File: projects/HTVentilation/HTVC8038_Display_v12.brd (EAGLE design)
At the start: 80.6 x 58.7 mm, 34 parts, among them IC1 7805T

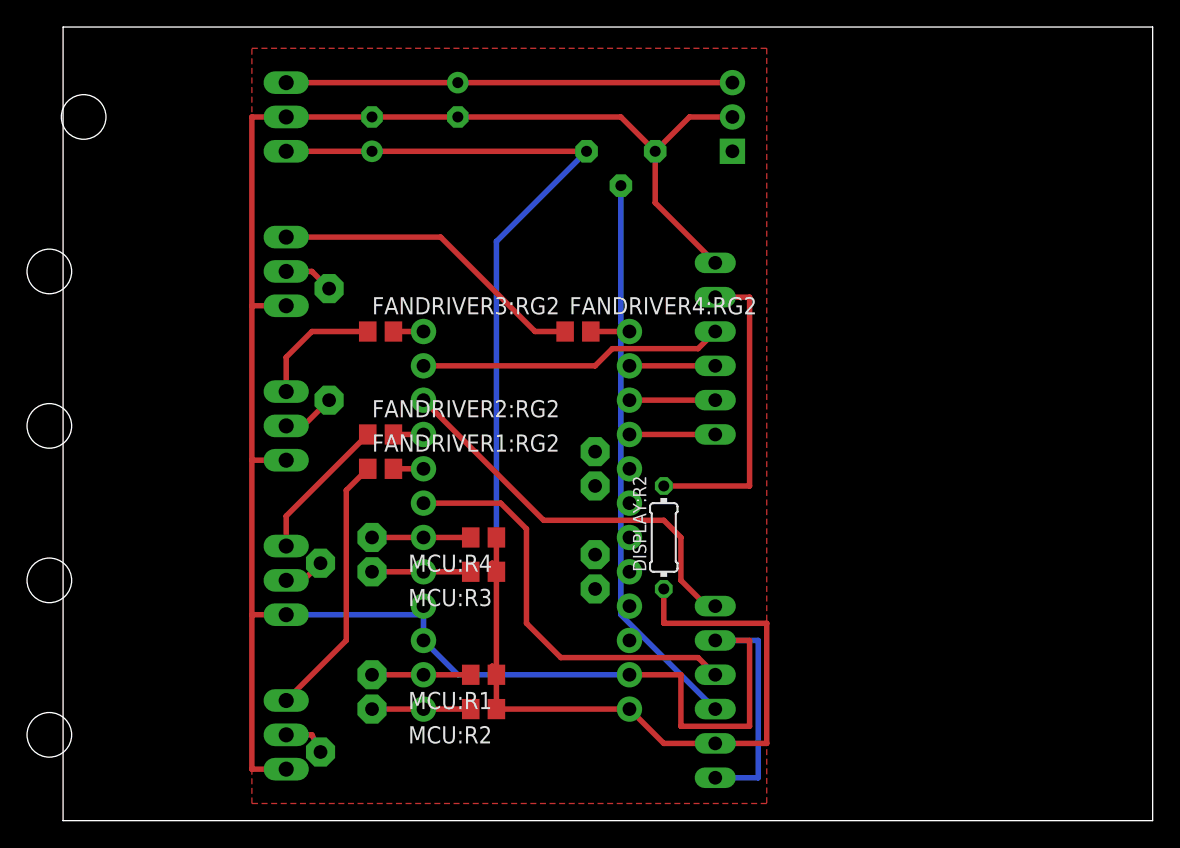
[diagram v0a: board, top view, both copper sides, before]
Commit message: cleanup
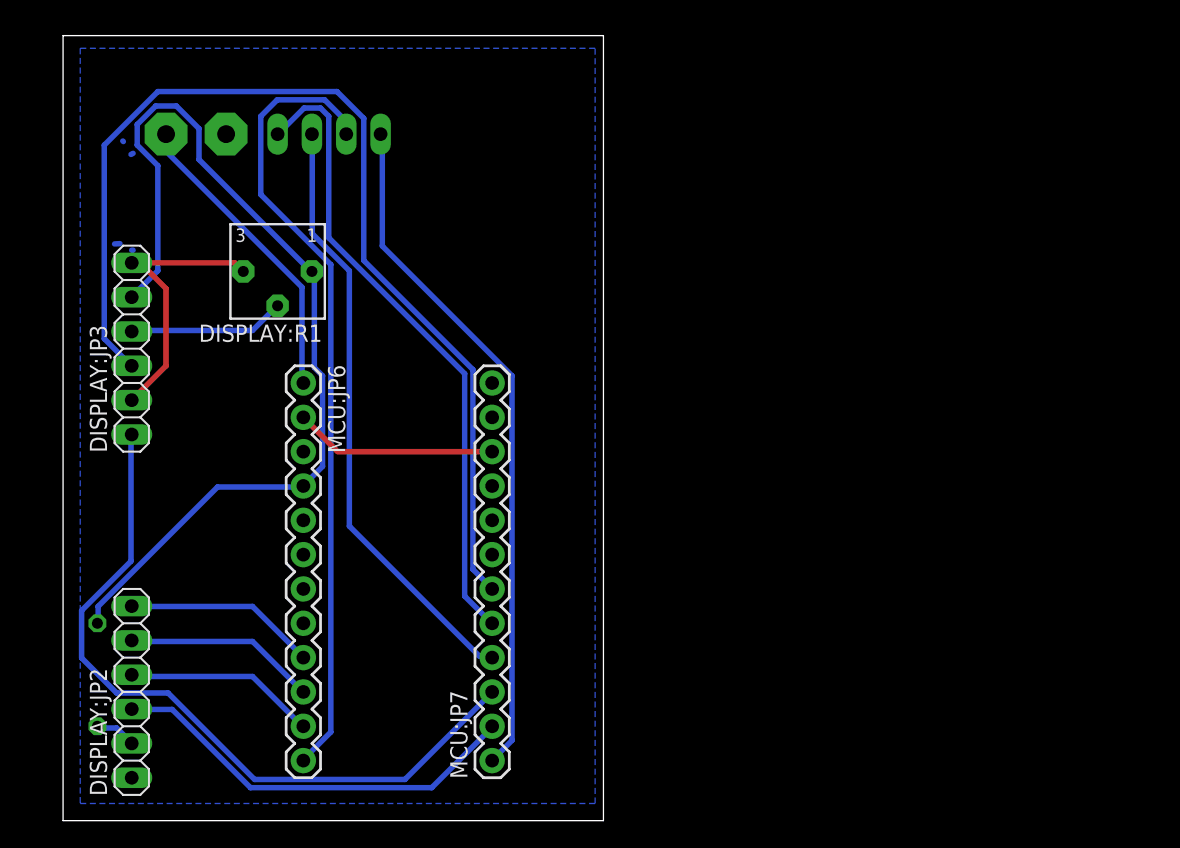
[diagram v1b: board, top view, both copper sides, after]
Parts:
- removed C1: 0.33uF, rcl:E2,5-6
- removed C2: 0.1uF, rcl:E2,5-6
- removed CONNECTORS_BOARD1:PAD1, CONNECTORS_BOARD1:PAD10, CONNECTORS_BOARD1:PAD11, CONNECTORS_BOARD1:PAD12, CONNECTORS_BOARD1:PAD2, CONNECTORS_BOARD1:PAD3, CONNECTORS_BOARD1:PAD4, CONNECTORS_BOARD1:PAD5, CONNECTORS_BOARD1:PAD6, CONNECTORS_BOARD1:PAD7, CONNECTORS_BOARD1:PAD8, CONNECTORS_BOARD1:PAD9: (no value), wirepad:2,15/1,0
- removed FANDRIVER1:RG2, FANDRIVER2:RG2, FANDRIVER3:RG2, FANDRIVER4:RG2: 1K, rcl:R0805
- removed FANDRIVER1:T1_1, FANDRIVER2:T1_1, FANDRIVER3:T1_1, FANDRIVER4:T1_1: TIP120, transistor-power:TO220AH
- removed IC1: 7805T, linear:TO220H
- removed JP1: (no value), SparkFun-Connectors:MOLEX-1X3
- removed MCU:R1, MCU:R2, MCU:R3, MCU:R4: 10K, rcl:R0805
- added +12V1, AGND9: (no value), wirepad:3,17/1,3
- added MCU:JP1: (no value), pinhead:1X04
- moved DISPLAY:JP2 50.1 mm to (5.08, 9.53), flipped to the top, turned to 90 degrees
- moved DISPLAY:JP3 50.1 mm to (5.08, 34.9), flipped to the top, turned to 90 degrees
- moved DISPLAY:R2 43.1 mm to (2.54, 10.8), flipped to the bottom, turned to 270 degrees
- moved MCU:JP6 34.1 mm to (17.8, 32.4), flipped to the top, turned to 270 degrees
- moved MCU:JP7 32.2 mm to (31.8, 4.45), flipped to the top, turned to 90 degrees
- moved DISPLAY:R1 26.9 mm to (15.9, 40.6), flipped to the top
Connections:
- removed net FANDRIVER1:N$10: FANDRIVER1:RG2.1, FANDRIVER1:T1_1.B
- removed net FANDRIVER2:N$10: FANDRIVER2:RG2.1, FANDRIVER2:T1_1.B
- removed net FANDRIVER3:N$10: FANDRIVER3:RG2.1, FANDRIVER3:T1_1.B
- removed net FANDRIVER4:N$10: FANDRIVER4:RG2.1, FANDRIVER4:T1_1.B
- removed net MCU:5VOUT: MCU:JP6.4
- removed net N$10: CONNECTORS_BOARD1:PAD10.1, FANDRIVER3:T1_1.C
- removed net N$11: CONNECTORS_BOARD1:PAD8.1, FANDRIVER2:T1_1.C
- removed net N$12: CONNECTORS_BOARD1:PAD6.1, FANDRIVER1:T1_1.C
- removed net N$9: CONNECTORS_BOARD1:PAD12.1, FANDRIVER4:T1_1.C
- net +5V: now also MCU:JP6.4; no longer C2.+, IC1.3, MCU:JP6.1, MCU:R1.1, MCU:R2.1, MCU:R3.1, MCU:R4.1
- net A0: no longer CONNECTORS_BOARD1:PAD1.1
- net A1: no longer CONNECTORS_BOARD1:PAD2.1
- net A2: no longer CONNECTORS_BOARD1:PAD3.1
- net A3: no longer CONNECTORS_BOARD1:PAD4.1
- net AGND: now also AGND9.1; no longer C1.-, C2.-, FANDRIVER1:T1_1.E, FANDRIVER2:T1_1.E, FANDRIVER3:T1_1.E, FANDRIVER4:T1_1.E, IC1.2, JP1.2
- net N$21: now also MCU:JP1.4; no longer FANDRIVER1:RG2.2
- net N$22: now also MCU:JP1.3; no longer FANDRIVER2:RG2.2
- net N$23: now also MCU:JP1.1; no longer FANDRIVER3:RG2.2
- net N$37: now also MCU:JP1.2; no longer FANDRIVER4:RG2.2
- net TACH0: no longer CONNECTORS_BOARD1:PAD5.1, MCU:R4.2
- net TACH1: no longer CONNECTORS_BOARD1:PAD7.1, MCU:R3.2
- net TACH2: no longer CONNECTORS_BOARD1:PAD9.1, MCU:R2.2
- net TACH3: no longer CONNECTORS_BOARD1:PAD11.1, MCU:R1.2
- net VCC: now also +12V1.1, MCU:JP6.1; no longer C1.+, IC1.1, JP1.3
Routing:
- net AGND: track 173.9 -> 39.4 mm
- net N$37: track 2.86 -> 59.1 mm
- net N$23: track 2.23 -> 51.0 mm
- net N$1: track 30.9 -> 77.6 mm
- net N$21: track 2.23 -> 47.4 mm
- net N$22: track 2.23 -> 44.8 mm
- net +5V: track 110.1 -> 71.1 mm
- net DISPLAY:N$1: track 41.6 -> 11.6 mm
- net N$2: track 29.8 -> 54.9 mm
- net FANDRIVER4:N$10: track 23.5 -> 0.00 mm
- net DISPLAY:N$2: track 22.9 -> 3.11 mm
- net FANDRIVER1:N$10: track 19.6 -> 0.00 mm
- net FANDRIVER2:N$10: track 10.8 -> 0.00 mm
- net VCC: track 33.0 -> 22.6 mm
- net FANDRIVER3:N$10: track 9.36 -> 0.00 mm
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- added copper zone on layer 16, net AGND
- removed copper zone on layer 1, net _GND
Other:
- board size 80.6 x 58.7 mm -> 40 x 58.1 mm
